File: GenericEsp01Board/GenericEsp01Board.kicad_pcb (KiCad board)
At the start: 2 copper layers, 46.4 x 26.7 mm, 13 parts, among them J1 DC IN, J2 5vSerial, J3 IO0, J4 IO2, U1 ESP, U2 AMS1117

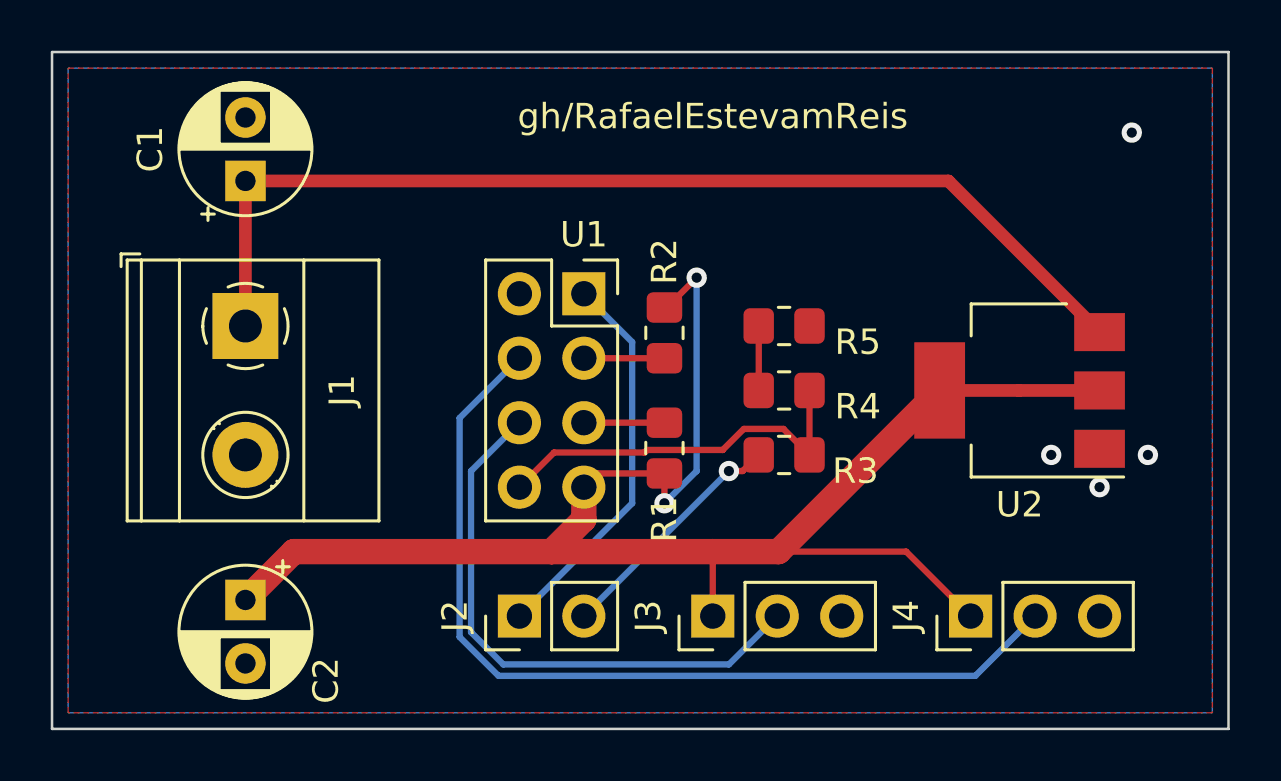
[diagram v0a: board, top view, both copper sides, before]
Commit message: V1
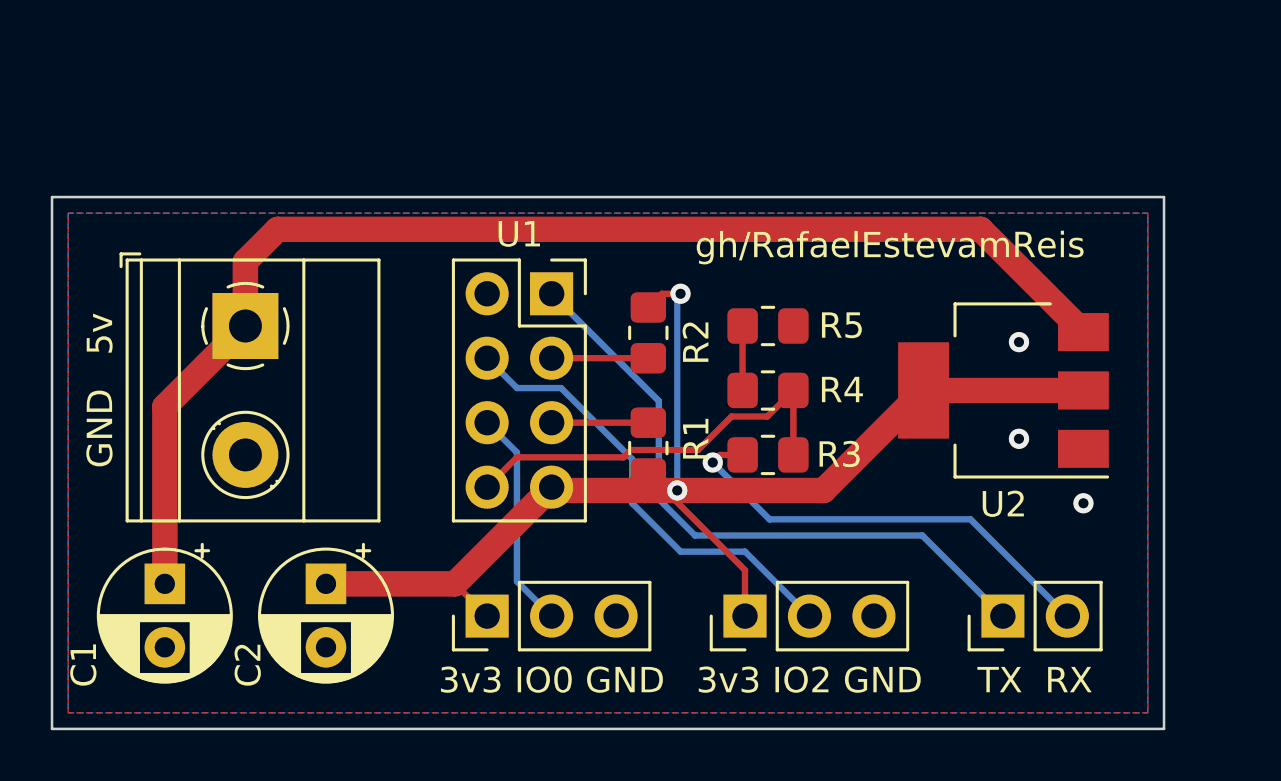
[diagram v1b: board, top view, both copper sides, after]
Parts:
- removed J2: 5vSerial, Connector_PinHeader_2.54mm:PinHeader_1x02_P2.54mm_Vertical
- removed J3: IO0, Connector_PinHeader_2.54mm:PinHeader_1x03_P2.54mm_Vertical
- added 3v3 IO0 GND: IO0, Connector_PinHeader_2.54mm:PinHeader_1x03_P2.54mm_Vertical, F.Cu at (106.7, 116.8)
- added TX  RX: 5vSerial, Connector_PinHeader_2.54mm:PinHeader_1x02_P2.54mm_Vertical, F.Cu at (127.0, 116.8)
- 3v3 IO2 GND: renamed from J4
- GND   5v: renamed from J1
- moved C1 16.2 mm to (94.0, 115.6), turned to 270 degrees
- moved 3v3 IO2 GND 8.89 mm to (116.8, 116.8)
- moved C2 3.24 mm to (100.3, 115.6)
- moved U1 1.27 mm to (109.2, 104.1)
- moved R1 0.64 mm to (113.0, 110.2)
- moved R2 0.64 mm to (113.0, 105.7)
- moved R3 0.63 mm to (117.7, 110.5)
- moved R4 0.63 mm to (117.7, 108.0)
- moved R5 0.63 mm to (117.7, 105.4)
- moved U2 0.63 mm to (127.0, 108.0)
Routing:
- net /GPIO2: track 36.2 -> 17.9 mm
- net /3v3: track 67.0 -> 52.1 mm
- net /GPIO0: track 22.4 -> 8.67 mm
- net /3v3_TX: track 15.3 -> 25.3 mm
- net Net-(J2-Pad2): track 9.52 -> 17.8 mm
- net /DC_IN: track 41.8 -> 49.2 mm
- net /3v3_RX: track 15.3 -> 16.2 mm
- net Net-(R2-Pad1): track 3.18 -> 3.81 mm
- net Net-(R1-Pad1): track 3.18 -> 3.81 mm
- net GND: vias 4 -> 3
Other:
- board size 46.4 x 26.7 mm -> 43.8 x 21 mm
